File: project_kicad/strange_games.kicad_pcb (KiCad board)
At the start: 2 copper layers, 330 x 247.5 mm, 118 parts, among them J1 Display, M1 Motor_DC, Q1 Si2302A, Q2 Q_Photo, Q3 Si2302A, Q4 Q_Photo, SW1 SW_Push, SW10 SW_Push, SW2 SW_Push, SW3 SW_Push, SW4 SW_Push, SW5 SW_Push, SW6 SW_Push, SW7 SW_Push, SW8 SW_Push, SW9 SW_Push, U1 charge controller, U2 boost converter, U3 LDL1117S33R, U4 ESP32-DEVKIT-V1, U5 TMP112xxDRL, U6 vibrating_sensor, U7 LSM6DS3, U8 MQ-135 gas sensor

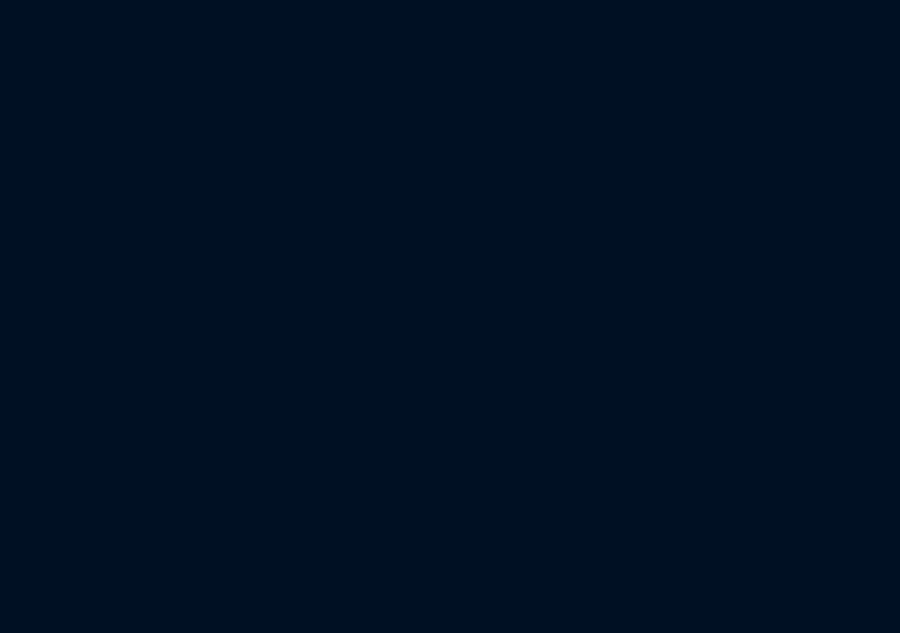
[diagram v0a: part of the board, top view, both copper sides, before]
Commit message: code changes
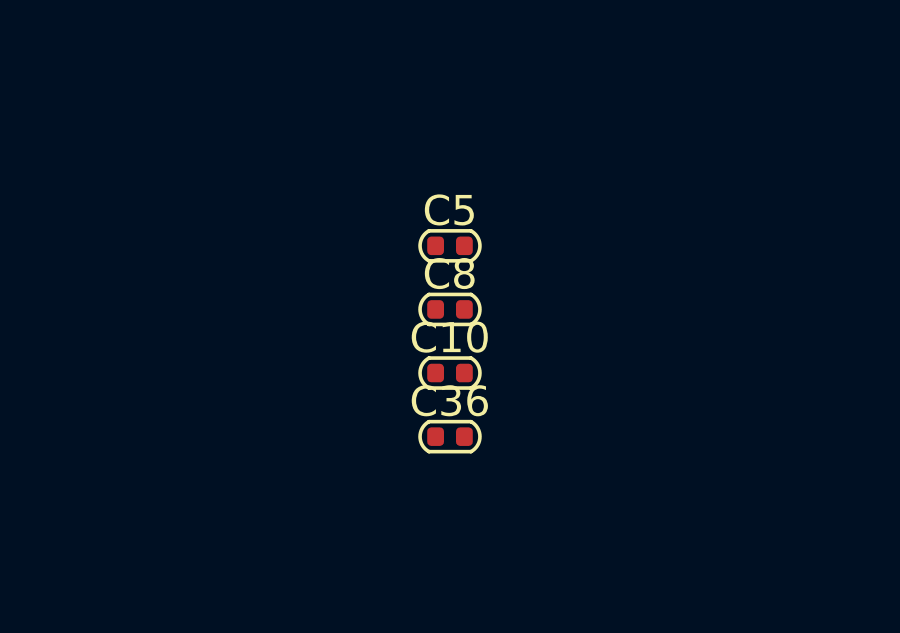
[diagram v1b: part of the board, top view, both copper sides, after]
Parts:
- added C10: C_Generic, PCM_Capacitor_SMD_AKL:C_0402_1005Metric, F.Cu at (338.9, 97.2)
- added C36: C_Generic, PCM_Capacitor_SMD_AKL:C_0402_1005Metric, F.Cu at (338.9, 99.4)
- added C5: C_Generic, PCM_Capacitor_SMD_AKL:C_0402_1005Metric, F.Cu at (338.9, 93.0)
- added C8: C_Generic, PCM_Capacitor_SMD_AKL:C_0402_1005Metric, F.Cu at (338.9, 95.1)
